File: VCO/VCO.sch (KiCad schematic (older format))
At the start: 51 parts, among them J1 EuroPower, J2 CV, J3 Triangle, J4 Square, J5 CV3, J6 Ramp, Q1 BC547, Q2 BC547, Q3 BC547, Q4 MMDT3904, Q5 BC547, U1 TL082, U2 TL082, U3 TL082

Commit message: VCO PCB
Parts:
- R18: footprint Resistor_THT:R_Axial_DIN0204_L3.6mm_D1.6mm_P7.62mm_Horizontal -> Resistor_THT:R_Axial_DIN0204_L3.6mm_D1.6mm_P2.54mm_Vertical
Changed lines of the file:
@@
 F 0 "R18" V 5650 950 50  0000 C CNN
 F 1 "22k" V 5750 950 50  0000 C CNN
-F 2 "Resistor_THT:R_Axial_DIN0204_L3.6mm_D1.6mm_P7.62mm_Horizontal" V 5680 950 50  0001 C CNN
+F 2 "Resistor_THT:R_Axial_DIN0204_L3.6mm_D1.6mm_P2.54mm_Vertical" V 5680 950 50  0001 C CNN
 F 3 "~" H 5750 950 50  0001 C CNN
 	1    5750 950

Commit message: VCO - Nice schematic
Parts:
- removed J1: EuroPower, Connector_IDC:IDC-Header_2x05_P2.54mm_Vertical, symbol Connector_Generic:Conn_02x05_Odd_Even
- removed J5: CV3, Connector_PinHeader_2.54mm:PinHeader_1x01_P2.54mm_Vertical, symbol Connector:Conn_01x01_Female
- removed J6: Ramp, Connector_PinHeader_2.54mm:PinHeader_1x01_P2.54mm_Vertical, symbol Connector:Conn_01x01_Female
- added D1, D2: LED, LED_SMD:LED_1206_3216Metric_ReverseMount_Hole1.8x2.4mm, symbol Device:LED
- added D3, D4: LED, LED_SMD:LED_1206_3216Metric_Castellated, symbol Device:LED
- added H1, H2: Mounting_Holes, Kosmo_panel:Kosmo_Panel_Dual_Mounting_Holes, symbol Kosmo:Mounting_Holes
- added J1: EuroPower, telec:EuroPower, symbol Connector:Screw_Terminal_01x03
- added J3: CV PWM, telec:JackHole, symbol Connector:AudioJack3_Switch
- added J5: PWM, telec:JackHole, symbol Connector:AudioJack3_Switch
- added J7: Ramp, telec:JackHole, symbol Connector:AudioJack3_Switch
- added LOGO1: telec, logo:telec-16, symbol logo:Logo_telec
- added R1: 130k, Resistor_THT:R_Axial_DIN0204_L3.6mm_D1.6mm_P7.62mm_Horizontal, symbol Device:R
- added R26, R27, R28, R29: 1k, Resistor_SMD:R_1206_3216Metric_Pad1.42x1.75mm_HandSolder, symbol Device:R
- added R30, R31: 2k2, Resistor_SMD:R_1206_3216Metric_Pad1.42x1.75mm_HandSolder, symbol Device:R
- added R32, R33: 1k5, Resistor_SMD:R_1206_3216Metric_Pad1.42x1.75mm_HandSolder, symbol Device:R
- added R5: 47k, Resistor_SMD:R_1206_3216Metric_Pad1.42x1.75mm_HandSolder, symbol Device:R
- added R6: 4k7, Resistor_SMD:R_1206_3216Metric_Pad1.42x1.75mm_HandSolder, symbol Device:R
- added RV1, RV3: 100k, Potentiometer_THT:Potentiometer_Piher_T-16L_Single_Vertical_Hole, symbol Device:R_POT
- added TP1: CV3, Connector_PinHeader_2.54mm:PinHeader_1x01_P2.54mm_Vertical, symbol Connector:TestPoint
- added unit 2 of U1
- added unit 3 of U1
- added unit 2 of U4
- RV4: renamed from RV1; footprint Potentiometer_THT:Potentiometer_Runtron_RM-065_Vertical -> Potentiometer_THT:Potentiometer_Bourns_3299W_Vertical
- RV5: renamed from RV3; footprint Potentiometer_THT:Potentiometer_Runtron_RM-065_Vertical -> Potentiometer_THT:Potentiometer_Bourns_3299W_Vertical
- RV6: renamed from RV4; footprint Potentiometer_THT:Potentiometer_Runtron_RM-065_Vertical -> telec:Potentiometer_P3.81mmx5.12mm_Vertical
- renumbered C6 to C3, C3 to C4, C4 to C5, C7 to C6, C5 to C7, J3 to J6, Q4 to Q1, Q1 to Q3, Q3 to Q4, R18 to R10, R3 to R11, R19 to R12, R20 to R13, R21 to R14, R8 to R15, R22 to R16, R5 to R17, R6 to R18, R9 to R19, R1 to R2, R10 to R20, R11 to R21, R12 to R22, R13 to R23, R16 to R24, R17 to R25, R2 to R3, R14 to R8, R15 to R9, TP1 to TP2, TP2 to TP3, TP3 to TP4, U1 to U4
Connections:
- net labels added: CVP, Offset, PWM, PWM_level
- wire segments 158 -> 184
- no-connect marks 11 -> 22
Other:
- note added: "5V"
- note added: "CV mix"
- note added: "Exponentiator"
- note added: "Front Panel"
- note added: "Input"
- note added: "Output"
- note added: "PWM"
- note added: "Ramp"
- note added: "VCO"
- moved on the sheet: C1, C2, C3, C4, C5, C6, C7, J4, J6, JP1, Q1A, Q1B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

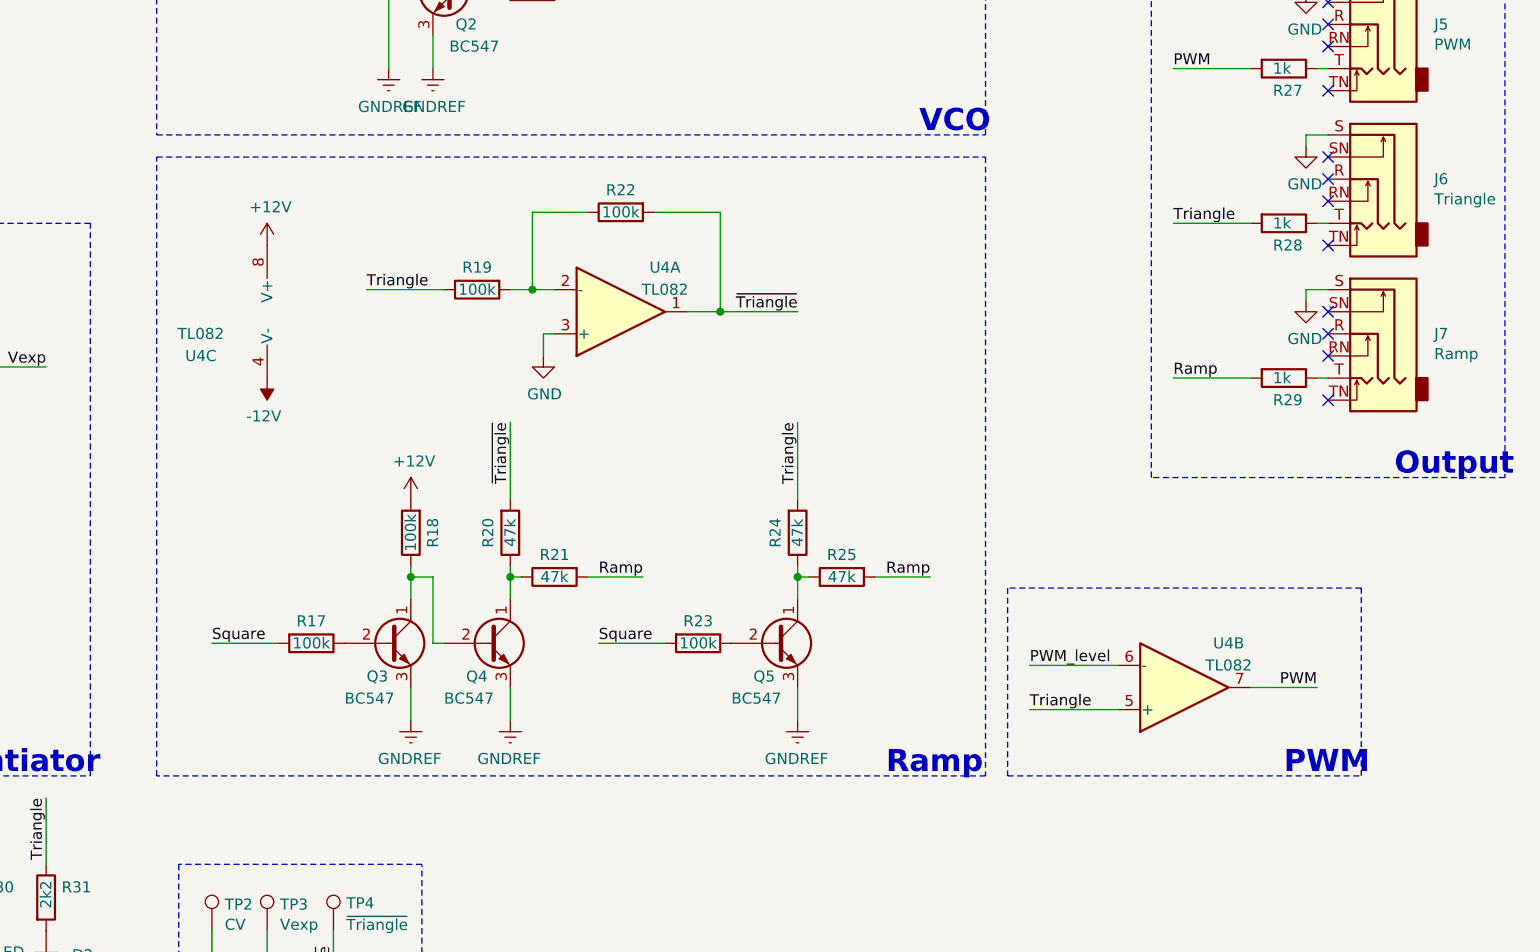
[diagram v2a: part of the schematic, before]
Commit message: VCO layout done!
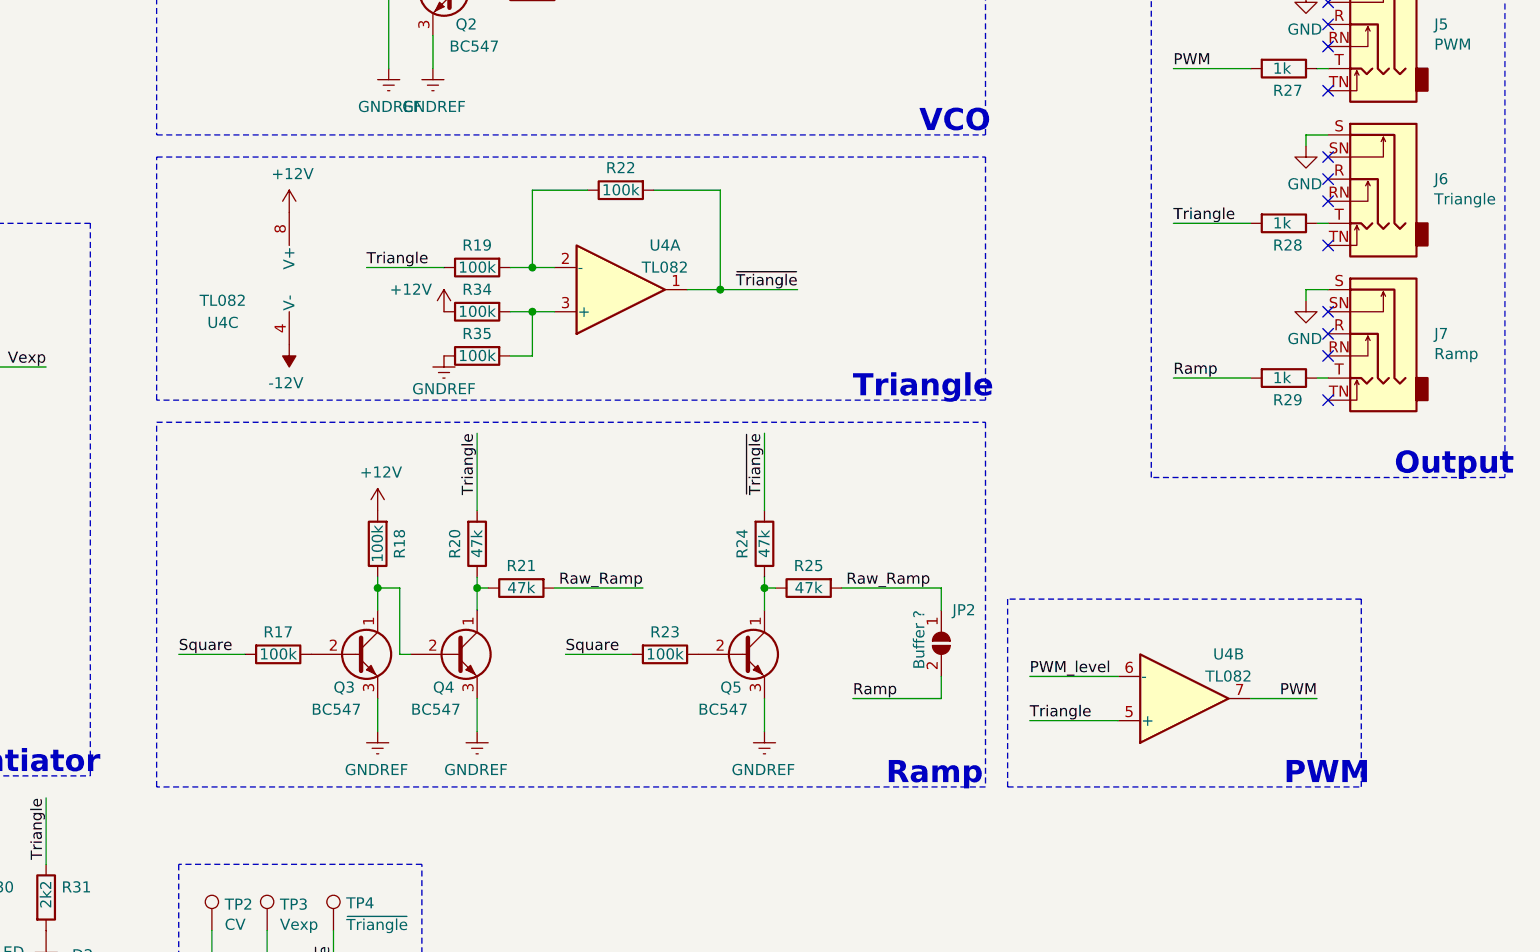
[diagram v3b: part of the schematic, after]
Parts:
- added JP2: Buffer ?, Jumper:SolderJumper-2_P1.3mm_Open_Pad1.0x1.5mm, symbol Jumper:SolderJumper_2_Open
- added R34, R35: 100k, Resistor_THT:R_Axial_DIN0204_L3.6mm_D1.6mm_P7.62mm_Horizontal, symbol Device:R
- R10: footprint Resistor_THT:R_Axial_DIN0204_L3.6mm_D1.6mm_P2.54mm_Vertical -> Resistor_THT:R_Axial_DIN0204_L3.6mm_D1.6mm_P7.62mm_Horizontal
- R5, R6: footprint Resistor_SMD:R_1206_3216Metric_Pad1.42x1.75mm_HandSolder -> Resistor_THT:R_Axial_DIN0204_L3.6mm_D1.6mm_P7.62mm_Horizontal
- U1: footprint Package_SO:SOIC-8_3.9x4.9mm_P1.27mm -> Package_DIP:DIP-8_W7.62mm_LongPads
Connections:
- net +12V: now also R34.1
- net GND: no longer U4.3 (+)
- net GNDREF: now also R35.1
- net Ramp: now also JP2.2 (B); no longer R21.2, R25.2
- net Triangle: now also R20.2; no longer R24.2
- net ~Triangle: now also R24.2; no longer R20.2
- new net: R34.2, R35.2, U4.3 (+)
- new net Raw_Ramp: JP2.1 (A), R21.2, R25.2
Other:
- note added: "Triangle"
- moved on the sheet: Q3, Q4, Q5, R17, R18, R19, R20, R21, R22, R23, R24, R25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
